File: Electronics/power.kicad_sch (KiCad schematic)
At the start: 25 parts, among them J1 USB_C_Receptacle_USB2.0, U2 MP2722, U3 TPD4E02B04DQA, U6 NCP186AMX330TAG

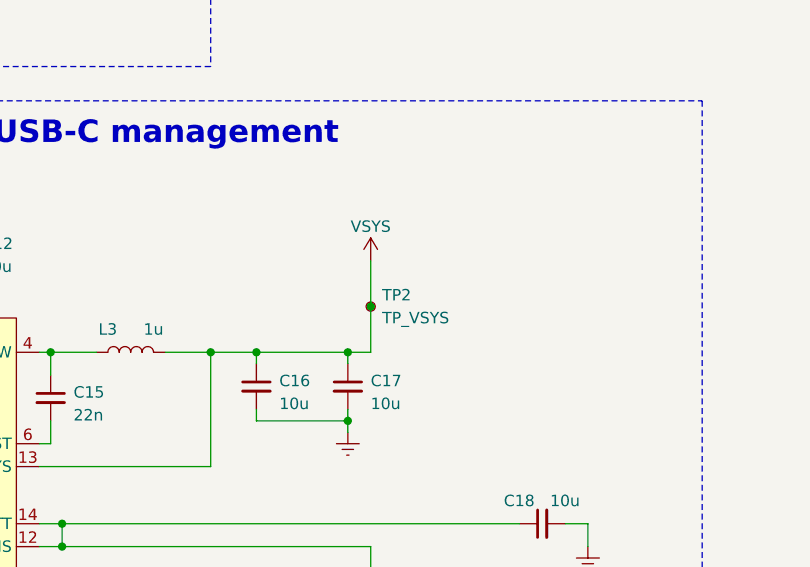
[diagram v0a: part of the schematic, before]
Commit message: Auto stash before merge of "latest" and "origin/latest"
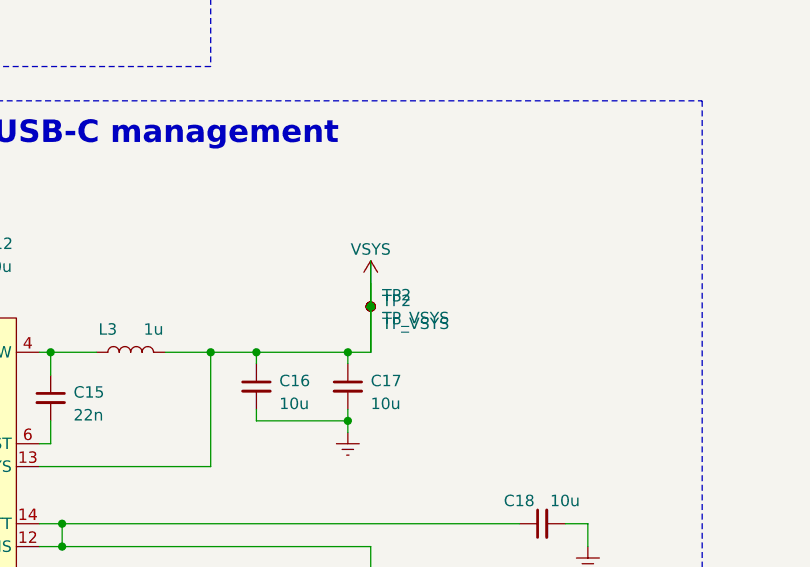
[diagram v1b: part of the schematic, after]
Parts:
- added TP2: TP_VSYS, TestPoint:TestPoint_Pad_D2.0mm, symbol Connector:TestPoint_Small
- J1: footprint Connector_USB:USB_C_Receptacle_Molex_105450-0101 -> USB4085:GCT_USB4085-GF-A_REVB
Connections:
- net VSYS: now also TP2.1
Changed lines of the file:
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@@
   (junction (at 74.93 140.97) (diameter 0) (color 0 0 0 0)
+  )
+  (junction (at 109.22 116.84) (diameter 0) (color 0 0 0 0)
   )
   (junction (at 34.29 163.83) (diameter 0) (color 0 0 0 0)
@@
     (stroke (width 0) (type default))
   )
+  (wire (pts (xy 109.22 116.84) (xy 109.22 114.3))
+    (stroke (width 0) (type default))
+  )
   (wire (pts (xy 58.42 67.31) (xy 74.93 67.31))
     (stroke (width 0) (type default))
@@
   )
   (wire (pts (xy 72.39 132.08) (xy 73.66 132.08))
+    (stroke (width 0) (type default))
+  )
+  (wire (pts (xy 109.22 121.92) (xy 109.22 116.84))
     (stroke (width 0) (type default))
   )
@@
       (effects (font (size 1.27 1.27)))
     )
-    (property "Footprint" "Connector_USB:USB_C_Receptacle_Molex_105450-0101" (at 39.37 59.69 0)
+    (property "Footprint" "USB4085:GCT_USB4085-GF-A_REVB" (at 39.37 59.69 0)
       (effects (font (size 1.27 1.27)) hide)
     )
@@
     )
   )
+  (symbol (lib_id "Connector:TestPoint_Small") (at 109.22 116.84 180) (unit 1)
+    (in_bom yes) (on_board yes) (dnp no) (fields_autoplaced)
+    (property "Reference" "TP2" (at 110.49 116.205 0)
+      (effects (font (size 1.27 1.27)) (justify right))
+    )
+    (property "Value" "TP_VSYS" (at 110.49 118.745 0)
+      (effects (font (size 1.27 1.27)) (justify right))
+    )
+    (property "Footprint" "TestPoint:TestPoint_Pad_D2.0mm" (at 104.14 116.84 0)
+      (effects (font (size 1.27 1.27)) hide)
+    )
+    (property "Datasheet" "~" (at 104.14 116.84 0)
+      (effects (font (size 1.27 1.27)) hide)
+    )
+    (pin "1")
+    (instances
+      (project "Aitken"
+        (path "/b70621e2-23d0-406f-b359-5b7c90496935/b637dce6-9faa-48d7-ac20-34c7af1e210c"
+          (reference "TP2") (unit 1)
+        )
+      )
+    )
+  )
   (symbol (lib_id "power:VBUS") (at 63.5 30.48 0) (unit 1)
     (in_bom yes) (on_board yes) (dnp no) (fields_autoplaced)
@@
     )
   )
-  (symbol (lib_id "more_power:VSYS") (at 109.22 111.76 0) (unit 1)
-    (in_bom yes) (on_board yes) (dnp no) (fields_autoplaced)
-    (property "Reference" "#PWR062" (at 109.22 115.57 0)
-      (effects (font (size 1.27 1.27)) hide)
-    )
-    (property "Value" "VSYS" (at 109.22 107.95 0)
+  (symbol (lib_id "more_power:VSYS") (at 109.22 114.3 0) (unit 1)
+    (in_bom yes) (on_board yes) (dnp no) (fields_autoplaced)
+    (property "Reference" "#PWR062" (at 109.22 118.11 0)
+      (effects (font (size 1.27 1.27)) hide)
+    )
+    (property "Value" "VSYS" (at 109.22 110.49 0)
       (effects (font (size 1.27 1.27)))
     )
-    (property "Footprint" "" (at 109.22 111.76 0)
-      (effects (font (size 1.27 1.27)) hide)
-    )
-    (property "Datasheet" "" (at 109.22 111.76 0)
-      (effects (font (size 1.27 1.27)) hide)
-    )
+    (property "Footprint" "" (at 109.22 114.3 0)
+      (effects (font (size 1.27 1.27)) hide)
+    )
+    (property "Datasheet" "" (at 109.22 114.3 0)
+      (effects (font (size 1.27 1.27)) hide)
+    )

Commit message: Changed USB port
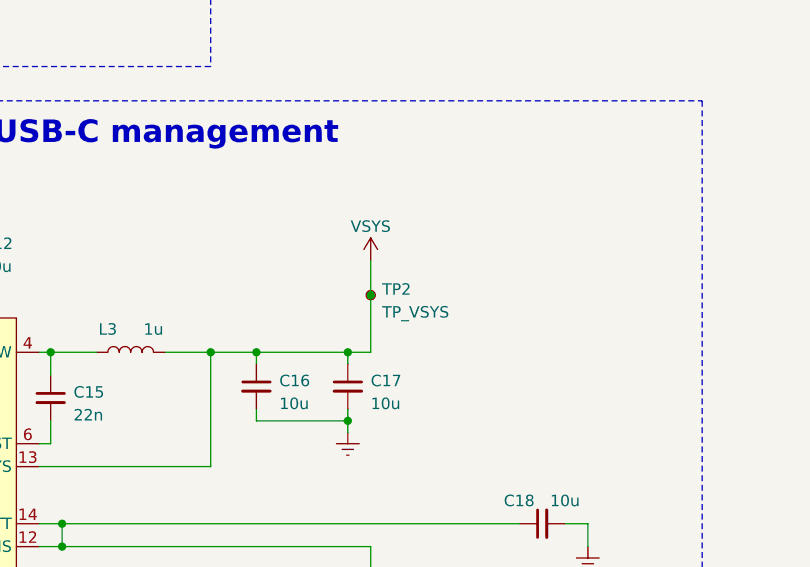
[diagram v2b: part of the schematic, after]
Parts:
- removed TP2 (x2): TP_VSYS, TestPoint:TestPoint_Pad_D2.0mm, symbol Connector:TestPoint_Small
- added TP2: TP_VSYS, TestPoint:TestPoint_Pad_D2.0mm, symbol Connector:TestPoint_Small
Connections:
- net VSYS: now also TP2.1
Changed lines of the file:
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@@
   (junction (at 74.93 140.97) (diameter 0) (color 0 0 0 0)
   )
-  (junction (at 109.22 116.84) (diameter 0) (color 0 0 0 0)
-  )
   (junction (at 34.29 163.83) (diameter 0) (color 0 0 0 0)
   )
   (junction (at 105.41 31.75) (diameter 0) (color 0 0 0 0)
   )
-  (junction (at 109.22 116.84) (diameter 0) (color 0 0 0 0)
-  )
   (junction (at 135.89 31.75) (diameter 0) (color 0 0 0 0)
   )
@@
   )
   (junction (at 113.03 31.75) (diameter 0) (color 0 0 0 0)
+  )
+  (junction (at 109.22 115.57) (diameter 0) (color 0 0 0 0)
   )
   (no_connect (at 27.94 82.55))
@@
     (stroke (width 0) (type default))
   )
-  (wire (pts (xy 109.22 116.84) (xy 109.22 114.3))
-    (stroke (width 0) (type default))
-  )
   (wire (pts (xy 58.42 67.31) (xy 74.93 67.31))
     (stroke (width 0) (type default))
@@
     (stroke (width 0) (type default))
   )
+  (wire (pts (xy 109.22 115.57) (xy 109.22 121.92))
+    (stroke (width 0) (type default))
+  )
   (wire (pts (xy 106.68 121.92) (xy 106.68 123.19))
     (stroke (width 0) (type default))
@@
     (stroke (width 0) (type default))
   )
-  (wire (pts (xy 109.22 116.84) (xy 109.22 121.92))
-    (stroke (width 0) (type default))
-  )
   (wire (pts (xy 106.68 130.81) (xy 106.68 129.54))
     (stroke (width 0) (type default))
@@
     (stroke (width 0) (type default))
   )
-  (wire (pts (xy 109.22 121.92) (xy 109.22 116.84))
+  (wire (pts (xy 109.22 111.76) (xy 109.22 115.57))
     (stroke (width 0) (type default))
   )
@@
   )
   (wire (pts (xy 52.07 33.02) (xy 52.07 44.45))
-    (stroke (width 0) (type default))
-  )
-  (wire (pts (xy 109.22 111.76) (xy 109.22 116.84))
     (stroke (width 0) (type default))
   )
@@
     )
   )
-  (symbol (lib_id "Connector:TestPoint_Small") (at 109.22 116.84 180) (unit 1)
-    (in_bom yes) (on_board yes) (dnp no) (fields_autoplaced)
-    (property "Reference" "TP2" (at 110.49 115.57 0)
-      (effects (font (size 1.27 1.27)) (justify right))
-    )
-    (property "Value" "TP_VSYS" (at 110.49 118.11 0)
-      (effects (font (size 1.27 1.27)) (justify right))
-    )
-    (property "Footprint" "TestPoint:TestPoint_Pad_D2.0mm" (at 104.14 116.84 0)
-      (effects (font (size 1.27 1.27)) hide)
-    )
-    (property "Datasheet" "~" (at 104.14 116.84 0)
-      (effects (font (size 1.27 1.27)) hide)
-    )
-    (pin "1")
-    (instances
-      (project "Aitken"
-        (path "/b70621e2-23d0-406f-b359-5b7c90496935/b637dce6-9faa-48d7-ac20-34c7af1e210c"
-          (reference "TP2") (unit 1)
-        )
-      )
-    )
-  )
   (symbol (lib_id "Device:C_Small") (at 96.52 125.73 0) (unit 1)
     (in_bom yes) (on_board yes) (dnp no) (fields_autoplaced)
@@
     )
   )
-  (symbol (lib_id "Connector:TestPoint_Small") (at 109.22 116.84 180) (unit 1)
-    (in_bom yes) (on_board yes) (dnp no) (fields_autoplaced)
-    (property "Reference" "TP2" (at 110.49 116.205 0)
-      (effects (font (size 1.27 1.27)) (justify right))
-    )
-    (property "Value" "TP_VSYS" (at 110.49 118.745 0)
-      (effects (font (size 1.27 1.27)) (justify right))
-    )
-    (property "Footprint" "TestPoint:TestPoint_Pad_D2.0mm" (at 104.14 116.84 0)
-      (effects (font (size 1.27 1.27)) hide)
-    )
-    (property "Datasheet" "~" (at 104.14 116.84 0)
-      (effects (font (size 1.27 1.27)) hide)
-    )
-    (pin "1")
-    (instances
-      (project "Aitken"
-        (path "/b70621e2-23d0-406f-b359-5b7c90496935/b637dce6-9faa-48d7-ac20-34c7af1e210c"
-          (reference "TP2") (unit 1)
+  (symbol (lib_id "more_power:VSYS") (at 109.22 111.76 0) (unit 1)
+    (in_bom yes) (on_board yes) (dnp no) (fields_autoplaced)
+    (property "Reference" "#PWR062" (at 109.22 115.57 0)
+      (effects (font (size 1.27 1.27)) hide)
+    )
+    (property "Value" "VSYS" (at 109.22 107.95 0)
+      (effects (font (size 1.27 1.27)))
+    )
+    (property "Footprint" "" (at 109.22 111.76 0)
+      (effects (font (size 1.27 1.27)) hide)
+    )
+    (property "Datasheet" "" (at 109.22 111.76 0)
+      (effects (font (size 1.27 1.27)) hide)
+    )
+    (pin "1")
+    (instances
+      (project "Aitken"
+        (path "/b70621e2-23d0-406f-b359-5b7c90496935/b637dce6-9faa-48d7-ac20-34c7af1e210c"
+          (reference "#PWR062") (unit 1)
         )
       )
@@
         (path "/b70621e2-23d0-406f-b359-5b7c90496935/b637dce6-9faa-48d7-ac20-34c7af1e210c"
           (reference "C18") (unit 1)
+        )
+      )
+    )
+  )
+  (symbol (lib_id "Connector:TestPoint_Small") (at 109.22 115.57 180) (unit 1)
+    (in_bom yes) (on_board yes) (dnp no) (fields_autoplaced)
+    (property "Reference" "TP2" (at 110.49 114.935 0)
+      (effects (font (size 1.27 1.27)) (justify right))
+    )
+    (property "Value" "TP_VSYS" (at 110.49 117.475 0)
+      (effects (font (size 1.27 1.27)) (justify right))
+    )
+    (property "Footprint" "TestPoint:TestPoint_Pad_D2.0mm" (at 104.14 115.57 0)
+      (effects (font (size 1.27 1.27)) hide)
+    )
+    (property "Datasheet" "~" (at 104.14 115.57 0)
+      (effects (font (size 1.27 1.27)) hide)
+    )
+    (pin "1")
+    (instances
+      (project "Aitken"
+        (path "/b70621e2-23d0-406f-b359-5b7c90496935/b637dce6-9faa-48d7-ac20-34c7af1e210c"
+          (reference "TP2") (unit 1)
         )
       )
@@
         )
       )
-    )
-  )
-  (symbol (lib_id "more_power:VSYS") (at 109.22 114.3 0) (unit 1)
-    (in_bom yes) (on_board yes) (dnp no) (fields_autoplaced)
-    (property "Reference" "#PWR062" (at 109.22 118.11 0)
-      (effects (font (size 1.27 1.27)) hide)
-    )
-    (property "Value" "VSYS" (at 109.22 110.49 0)
-      (effects (font (size 1.27 1.27)))
-    )
-    (property "Footprint" "" (at 109.22 114.3 0)
-      (effects (font (size 1.27 1.27)) hide)
-    )
-    (property "Datasheet" "" (at 109.22 114.3 0)
-      (effects (font (size 1.27 1.27)) hide)
-    )
-    (pin "1")
-    (instances
-      (project "Aitken"
-        (path "/b70621e2-23d0-406f-b359-5b7c90496935/b637dce6-9faa-48d7-ac20-34c7af1e210c"
-          (reference "#PWR062") (unit 1)
-        )
-      )
